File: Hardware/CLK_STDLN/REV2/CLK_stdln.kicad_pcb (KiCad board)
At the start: 2 copper layers, 63.9 x 67 mm, 43 parts, among them J1 Conn_01x04_Male, J2 Conn_Coaxial, J3 Conn_01x02, J4 Conn_02x20_Counter_Clockwise, Q1 BC547, Q2 BC547, Q3 BC547, SW1 SW_Push, SW2 SW_SPDT, SW3 SW_SPDT, U1 74LS08, U2 74LS04, U3 NE555, U4 NE555, U5 NE555

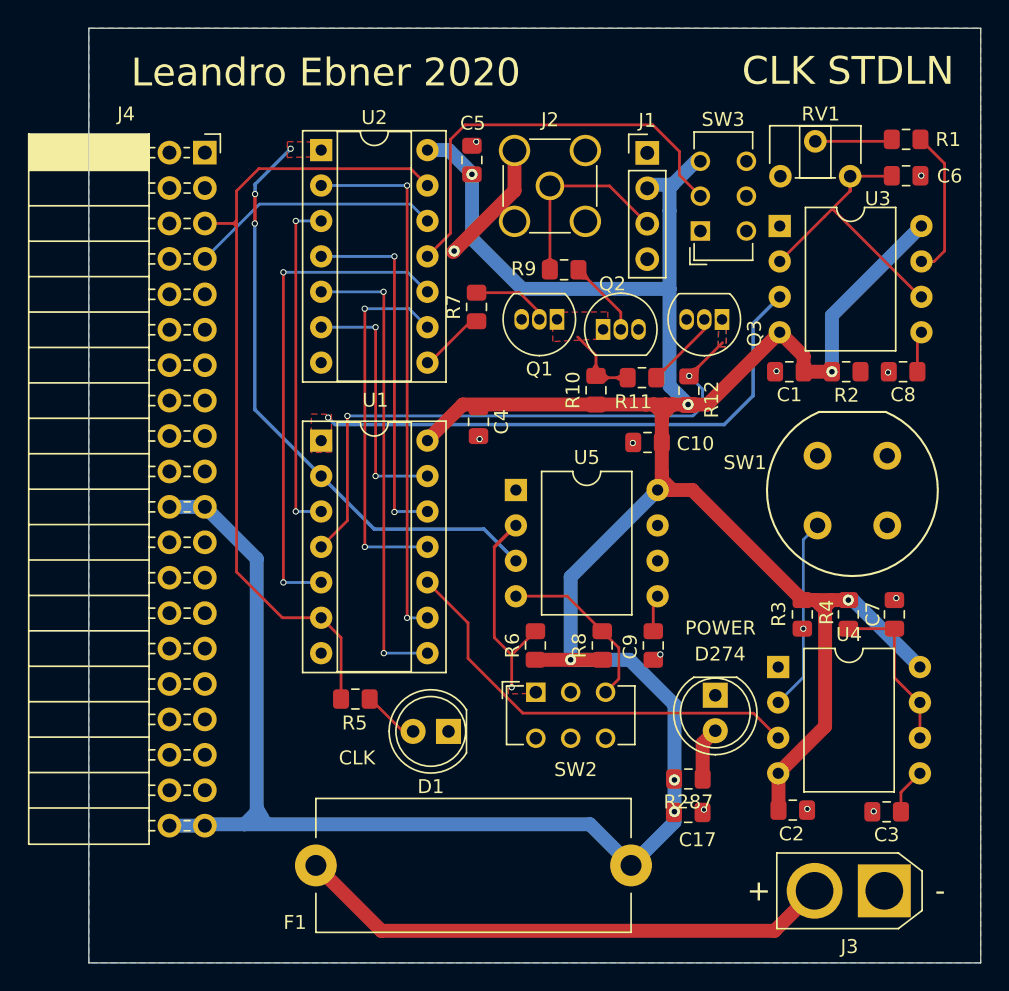
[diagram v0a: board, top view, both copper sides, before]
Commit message: 0047 | 0.5h | review ALU Module
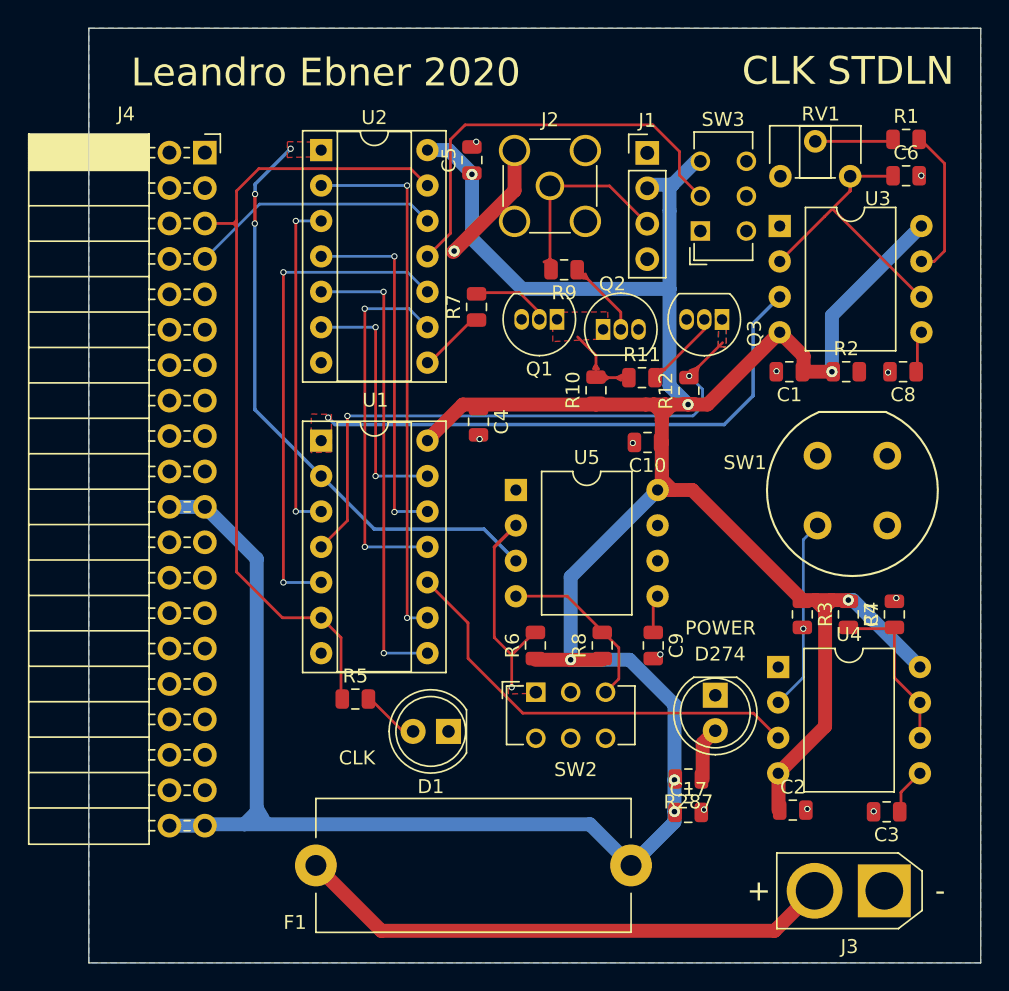
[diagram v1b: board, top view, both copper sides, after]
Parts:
- C1, C10, C17, C2, C3, C4, C5, C6, C7, C8, C9: footprint Capacitor_SMD:C_0805_2012Metric_Pad1.15x1.40mm_HandSolder -> Capacitor_SMD:C_0805_2012Metric
- R1, R10, R11, R12, R2, R287, R3, R4, R5, R6, R7, R8, R9: footprint Resistor_SMD:R_0805_2012Metric_Pad1.15x1.40mm_HandSolder -> Resistor_SMD:R_0805_2012Metric
